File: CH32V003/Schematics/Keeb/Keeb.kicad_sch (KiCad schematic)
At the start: 21 parts, among them P1 USB_C_Plug_USB2.0, SW1 SW_Push_45deg, SW2 SW_Push_45deg, SW3 SW_Push_45deg, SW4 SW_Push_45deg, U1 CH32V003F4P6, U2 TLV1117-33

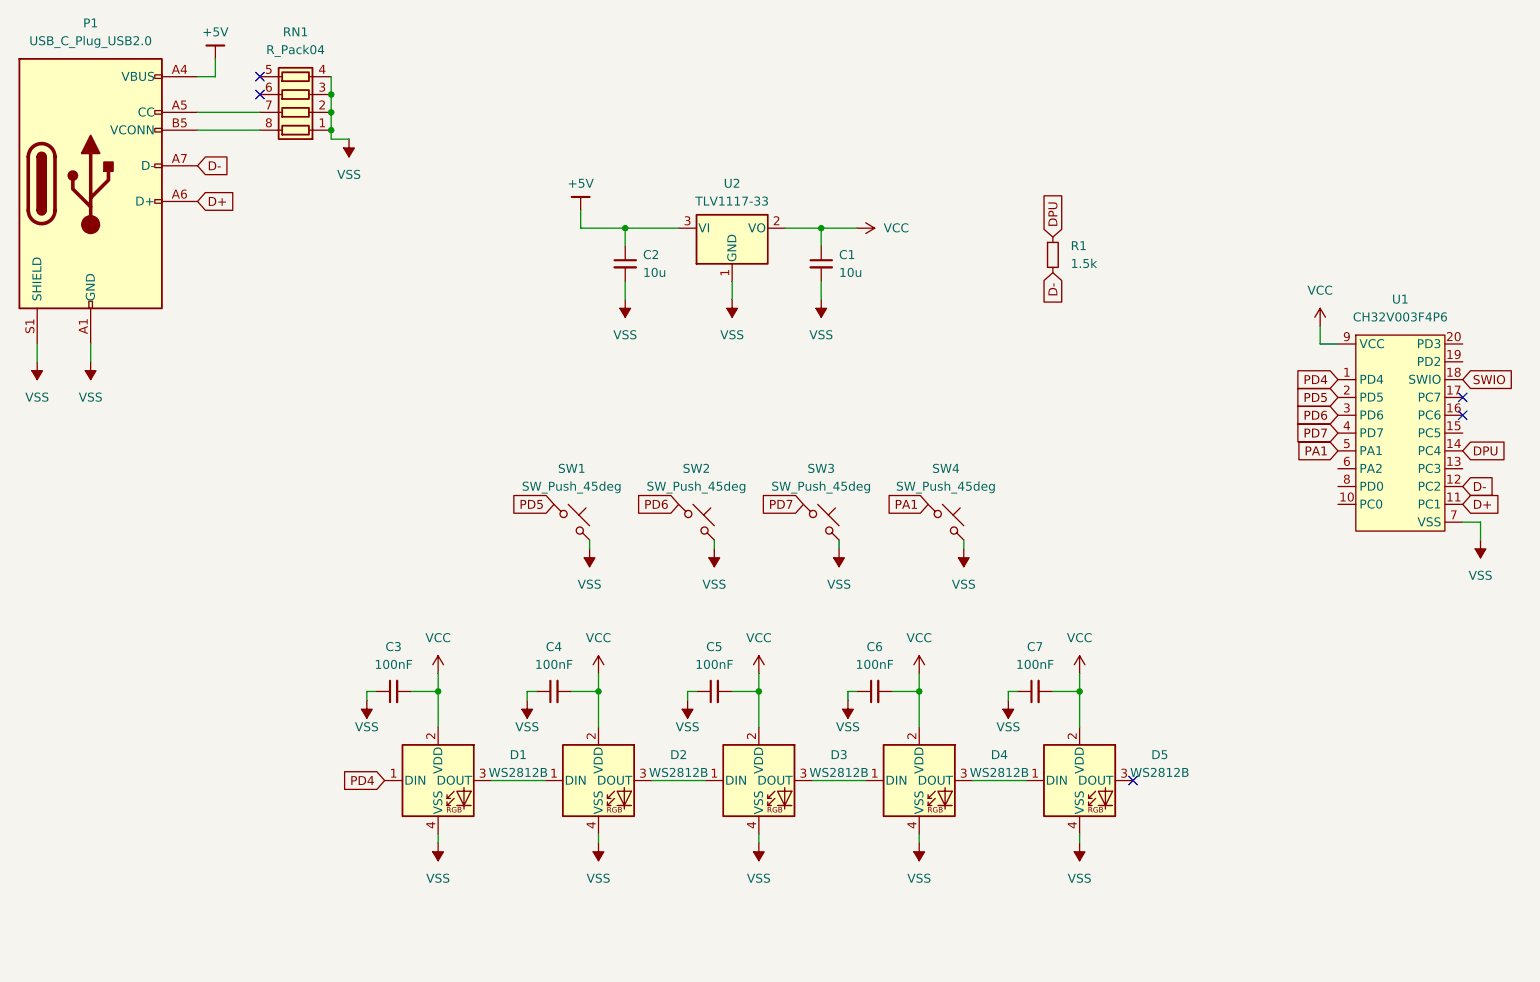
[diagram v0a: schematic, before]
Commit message: Ordered Keeb and K33b
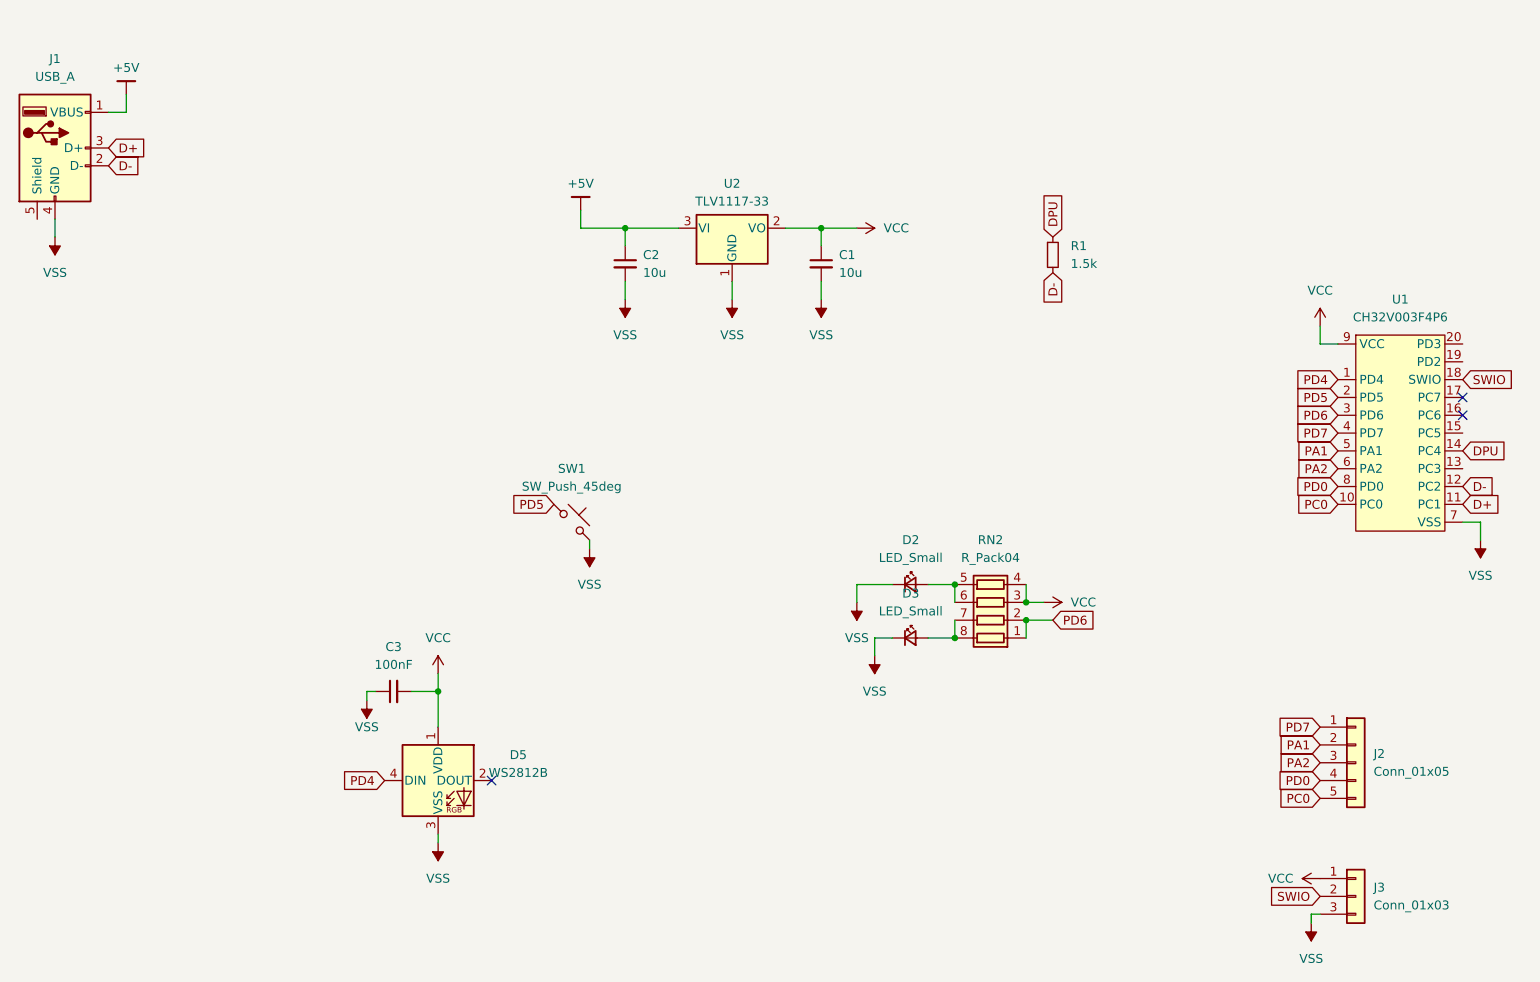
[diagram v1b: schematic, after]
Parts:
- removed C4, C5, C6, C7: 100nF, symbol Device:C_Small
- removed D1, D2, D3, D4: WS2812B, LED_SMD:LED_WS2812B_PLCC4_5.0x5.0mm_P3.2mm, symbol LED:WS2812B
- removed P1: USB_C_Plug_USB2.0, symbol Connector:USB_C_Plug_USB2.0
- removed RN1: R_Pack04, symbol Device:R_Pack04
- removed SW2, SW3, SW4: SW_Push_45deg, symbol Switch:SW_Push_45deg
- added D2, D3: LED_Small, LED_SMD:LED_0805_2012Metric, symbol Device:LED_Small
- added J1: USB_A, UL_USB:CONN-USB-A-PCB-TRACES, symbol Connector:USB_A
- added J2: Conn_01x05, Connector_PinHeader_2.54mm:PinHeader_1x05_P2.54mm_Vertical, symbol Connector_Generic:Conn_01x05
- added J3: Conn_01x03, Connector_PinHeader_2.54mm:PinHeader_1x03_P2.54mm_Vertical, symbol Connector_Generic:Conn_01x03
- added RN2: R_Pack04, Resistor_SMD:R_Array_Convex_4x0603, symbol Device:R_Pack04
- C1, C2, C3: footprint (none) -> Capacitor_SMD:C_0805_2012Metric
- D5: footprint LED_SMD:LED_WS2812B_PLCC4_5.0x5.0mm_P3.2mm -> cafebabe:SK6812-E_Reverse
- R1: footprint (none) -> Resistor_SMD:R_0805_2012Metric
- SW1: footprint (none) -> Button_Switch_Keyboard:SW_Cherry_MX_1.00u_PCB
- U1: footprint (none) -> Package_SO:TSSOP-20_4.4x6.5mm_P0.65mm
- U2: footprint (none) -> Package_TO_SOT_SMD:SOT-23-3
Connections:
- net +5V: now also J1.1 (VBUS)
- net D+: now also J1.3 (D+)
- net D-: now also J1.2 (D-)
- net PA1: now also J2.2 (Pin_2)
- net PD4: now also D5.4 (DIN)
- net PD6: now also RN2.1 (R1.1), RN2.2 (R2.1)
- net PD7: now also J2.1 (Pin_1)
- net SWIO: now also J3.2 (Pin_2)
- net VCC: now also D5.1 (VDD), J3.1 (Pin_1), RN2.3 (R3.1), RN2.4 (R4.1); no longer D5.2 (VDD)
- net VSS: now also D5.3 (VSS), D2.1 (K), D3.1 (K), J1.4 (GND), J3.3 (Pin_3); no longer D5.4 (VSS)
- net PC0: now reaches U1.10 (PC0)
- net PC0: now also J2.5 (Pin_5)
- net PA2: now reaches U1.6 (PA2)
- net PA2: now also J2.3 (Pin_3)
- net PD0: now reaches U1.8 (PD0)
- net PD0: now also J2.4 (Pin_4)
- new net: D2.2 (A), RN2.5 (R4.2), RN2.6 (R3.2)
- new net: D3.2 (A), RN2.7 (R2.2), RN2.8 (R1.2)
- no-connect marks 5 -> 3
